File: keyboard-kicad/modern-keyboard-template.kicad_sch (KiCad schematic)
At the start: 4 parts, among them J1 S2B-PH-K-S_LF__SN_, U1 nice_nano

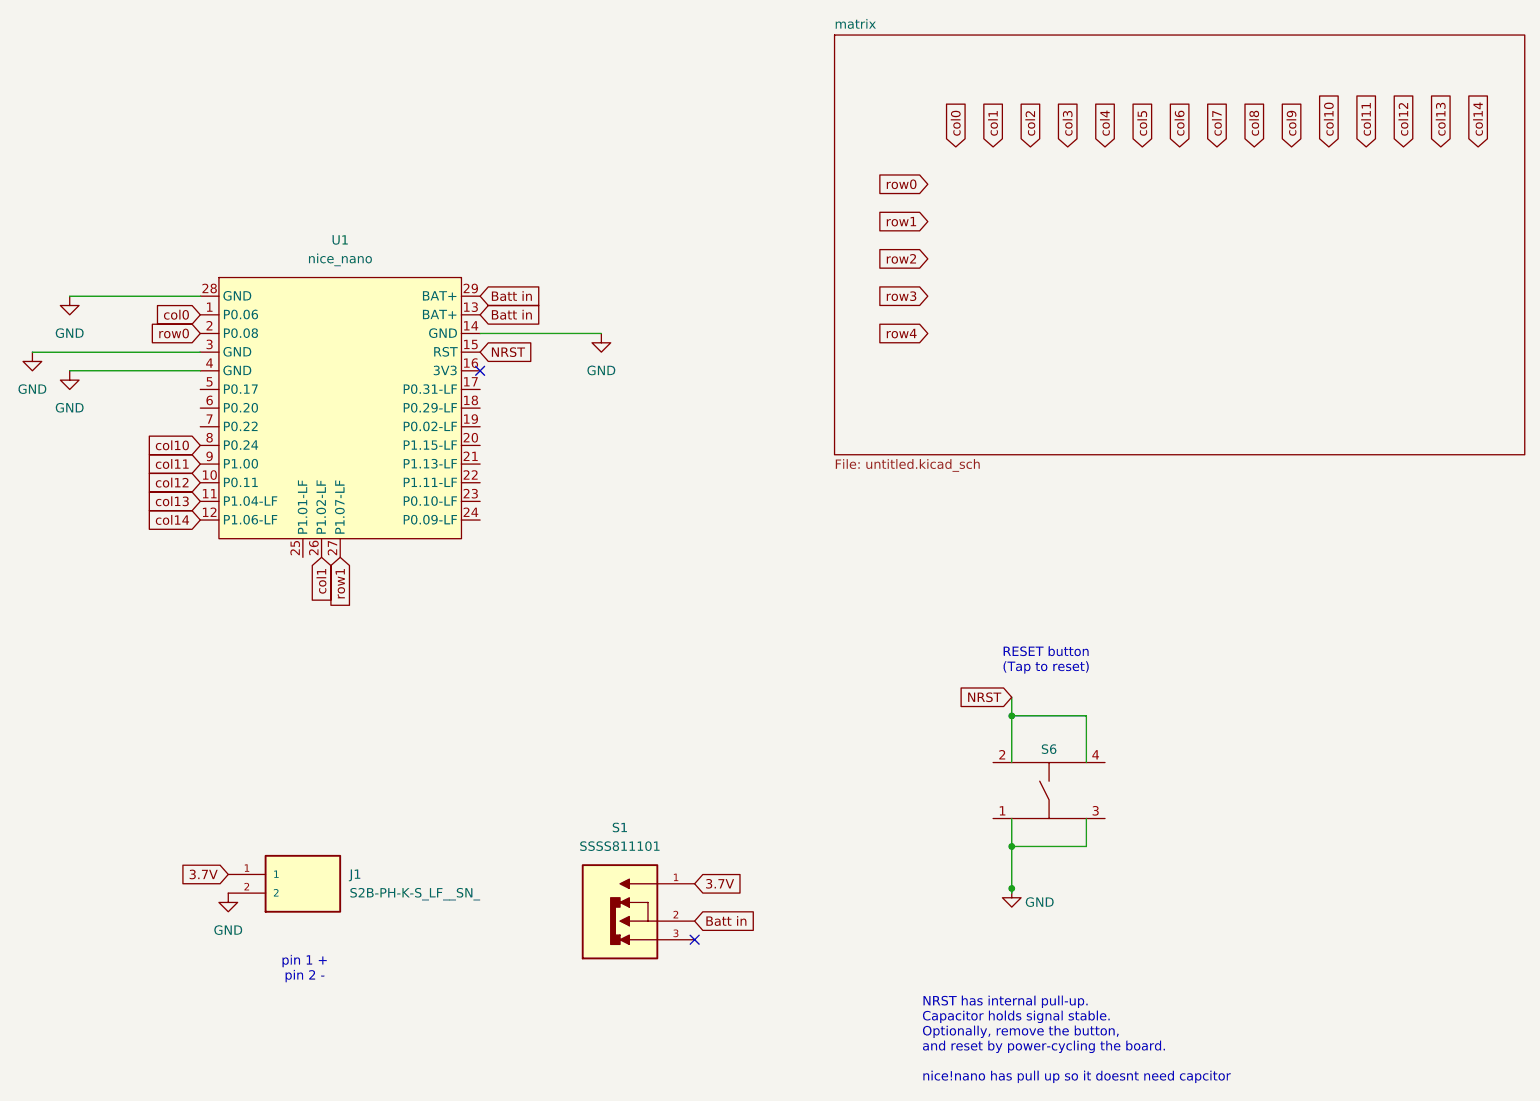
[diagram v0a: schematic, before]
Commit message: final kicad
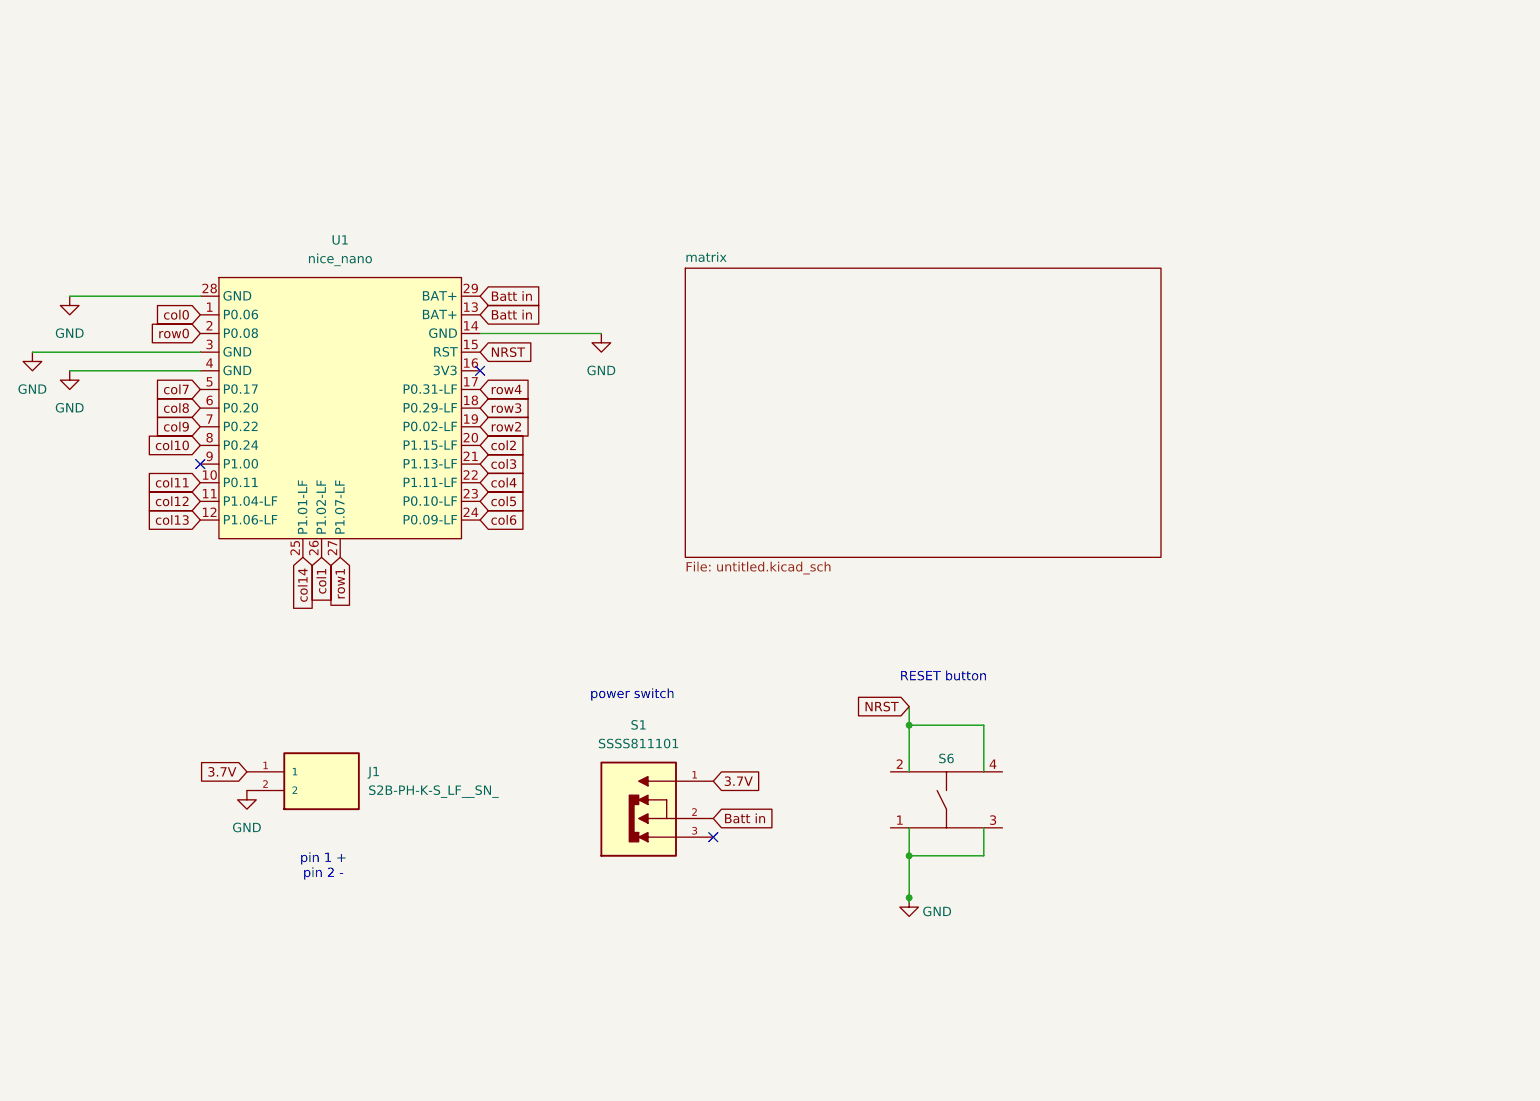
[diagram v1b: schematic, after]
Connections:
- net col11: now also U1.10 (P0.11); no longer U1.9 (P1.00)
- net col12: now also U1.11 (P1.04-LF); no longer U1.10 (P0.11)
- net col13: now also U1.12 (P1.06-LF); no longer U1.11 (P1.04-LF)
- net col14: now also U1.25 (P1.01-LF); no longer U1.12 (P1.06-LF)
- net col2: now also U1.20 (P1.15-LF)
- net col3: now also U1.21 (P1.13-LF)
- net col4: now also U1.22 (P1.11-LF)
- net col5: now also U1.23 (P0.10-LF)
- net col6: now also U1.24 (P0.09-LF)
- net col7: now also U1.5 (P0.17)
- net col8: now also U1.6 (P0.20)
- net col9: now also U1.7 (P0.22)
- net row2: now also U1.19 (P0.02-LF)
- net row3: now also U1.18 (P0.29-LF)
- net row4: now also U1.17 (P0.31-LF)
- no-connect marks 2 -> 3
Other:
- note added: "RESET button"
- note added: "power switch"
- note removed: "NRST has internal pull-up. Capacitor holds signal stable. Optionally, remove the button, and reset by power-cycling the board. nice!nano has pull up so it doesnt need capcitor"
- note removed: "RESET button (Tap to reset)"
- moved on the sheet: J1, S1, S6
